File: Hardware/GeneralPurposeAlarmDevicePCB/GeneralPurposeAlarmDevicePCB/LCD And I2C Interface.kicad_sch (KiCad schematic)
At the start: 18 parts, among them Q301 BSS138, U301 PCF8574AT, U302 LCD_20x4_Character-GPAD_SCH_L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

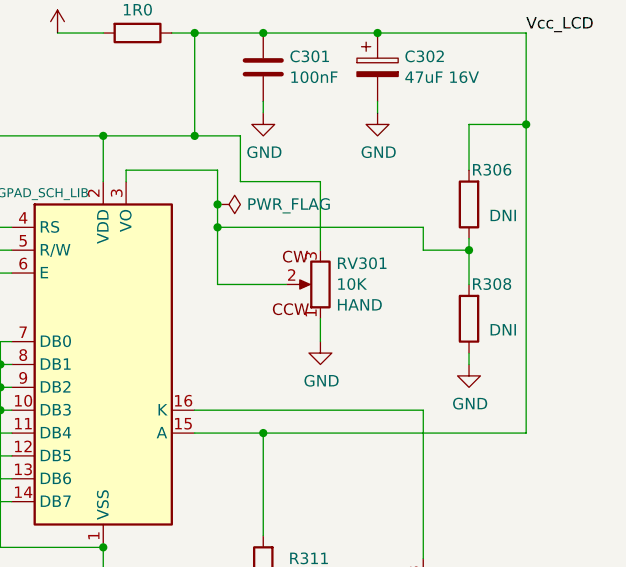
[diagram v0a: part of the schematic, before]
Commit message: Fix pot foot print, Add fifth mounting hole. Place all but UNO and test point.
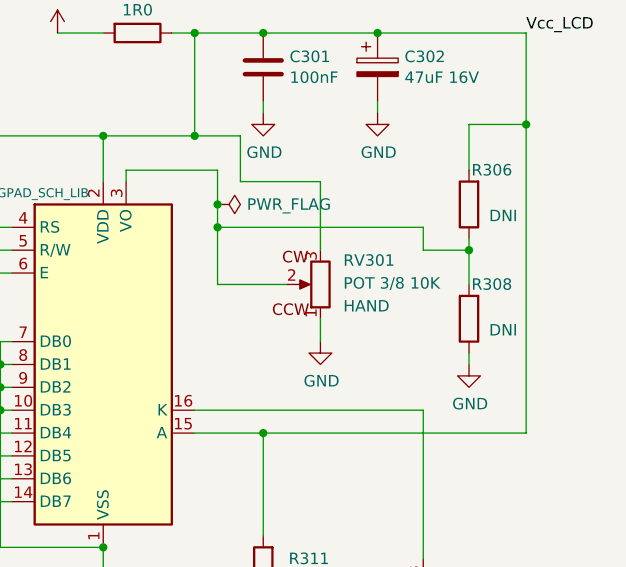
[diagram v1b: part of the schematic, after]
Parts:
- removed RV301: 10K, GeneralPurposeAlarmDevicePCB:Potentiometer_Bourns_3386P_Vertical, symbol GPAD_SCH_LIB:10K
- added RV301: POT 3/8 10K, GeneralPurposeAlarmDevicePCB:Potentiometer_Bourns_3386P_Vertical, symbol GPAD_SCH_LIB:POT 3/8 10K
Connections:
- net GND: now also RV301.1
- net Vcc_LCD: now also RV301.3
- net at R306.1, R308.2, U302.3 (VO): now also RV301.2
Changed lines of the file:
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@@
     (pin "1")
-  )
-  (symbol (lib_id "GPAD_SCH_LIB:10K") (at 209.55 68.58 180) (unit 1)
-    (in_bom yes) (on_board yes)
-    (property "Reference" "RV301" (id 0) (at 211.328 66.2686 0)
-      (effects (font (size 1.27 1.27)) (justify right))
-    )
-    (property "Value" "10K" (id 1) (at 211.328 68.58 0)
-      (effects (font (size 1.27 1.27)) (justify right))
-    )
-    (property "Footprint" "GeneralPurposeAlarmDevicePCB:Potentiometer_Bourns_3386P_Vertical" (id 2) (at 209.55 68.58 0)
-      (effects (font (size 1.27 1.27)) hide)
-    )
-    (property "Datasheet" "https://www.bourns.com/docs/Product-Datasheets/TC33.pdf" (id 3) (at 209.55 68.58 0)
-      (effects (font (size 1.27 1.27)) hide)
-    )
-    (property "Distributor 1" "JLCPCB" (id 4) (at 209.55 68.58 0)
-      (effects (font (size 1.27 1.27)) hide)
-    )
-    (property "Distributor 1 PN" "C58159" (id 5) (at 209.55 68.58 0)
-      (effects (font (size 1.27 1.27)) hide)
-    )
-    (property "Manufacturer" "BOURNS" (id 6) (at 209.55 68.58 0)
-      (effects (font (size 1.27 1.27)) hide)
-    )
-    (property "MPN" "3362P-1-103LF" (id 7) (at 209.55 68.58 0)
-      (effects (font (size 1.27 1.27)) hide)
-    )
-    (property "Assembly Type" "HAND" (id 8) (at 211.328 70.8914 0)
-      (effects (font (size 1.27 1.27)) (justify right))
-    )
-    (property "Manufacturier" "BOURNS" (id 9) (at 209.55 68.58 0)
-      (effects (font (size 1.27 1.27)) hide)
-    )
-    (pin "1")
-    (pin "2")
-    (pin "3")
   )
   (symbol (lib_id "power:PWR_FLAG") (at 167.64 49.53 0) (unit 1)
@@
     (pin "2")
   )
+  (symbol (lib_id "GPAD_SCH_LIB:POT 3/8 10K") (at 209.55 68.58 180) (unit 1)
+    (in_bom yes) (on_board yes) (fields_autoplaced)
+    (property "Reference" "RV301" (id 0) (at 212.09 65.9129 0)
+      (effects (font (size 1.27 1.27)) (justify right))
+    )
+    (property "Value" "POT 3/8 10K" (id 1) (at 212.09 68.4529 0)
+      (effects (font (size 1.27 1.27)) (justify right))
+    )
+    (property "Footprint" "GeneralPurposeAlarmDevicePCB:Potentiometer_Bourns_3386P_Vertical" (id 2) (at 209.55 68.58 0)
+      (effects (font (size 1.27 1.27)) hide)
+    )
+    (property "Datasheet" "https://www.bourns.com/docs/Product-Datasheets/3386.pdf" (id 3) (at 209.55 68.58 0)
+      (effects (font (size 1.27 1.27)) hide)
+    )
+    (property "Distributor 1" "JLCPCB" (id 4) (at 209.55 68.58 0)
+      (effects (font (size 1.27 1.27)) hide)
+    )
+    (property "Distributor 1 PN" "C116281" (id 5) (at 209.55 68.58 0)
+      (effects (font (size 1.27 1.27)) hide)
+    )
+    (property "Manufacturier" "BOURNS" (id 6) (at 209.55 68.58 0)
+      (effects (font (size 1.27 1.27)) hide)
+    )
+    (property "MPN" "3386P-1-103LF" (id 7) (at 209.55 68.58 0)
+      (effects (font (size 1.27 1.27)) hide)
+    )
+    (property "Assembly Type" "HAND" (id 8) (at 212.09 70.9929 0)
+      (effects (font (size 1.27 1.27)) (justify right))
+    )
+    (property "Distributor 2" "Digi-Key" (id 9) (at 209.55 68.58 0)
+      (effects (font (size 1.27 1.27)) hide)
+    )
+    (property "Distributor 2 PN" "3386P-103LF-ND" (id 10) (at 212.09 72.2629 0)
+      (effects (font (size 1.27 1.27)) (justify right) hide)
+    )
+    (property "Cost" "" (id 11) (at 209.55 68.58 0))
+    (pin "1")
+    (pin "2")
+    (pin "3")
+  )
   (symbol (lib_id "GPAD_SCH_LIB:LCD_20x4_Character-GPAD_SCH_LIB") (at 185.42 77.47 0) (unit 1)

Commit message: Delete lines related to the pot. The schematic now loads.
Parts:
- RV301: value POT 3/8 10K -> POT 0.375 10K; symbol GPAD_SCH_LIB:POT 3/8 10K -> GPAD_SCH_LIB:POT 0.375 10K
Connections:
- net GND: no longer RV301.1
- net Vcc_LCD: no longer RV301.3
- net at R306.1, R308.2, U302.3 (VO): no longer RV301.2
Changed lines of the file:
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@@
     (pin "2")
   )
-  (symbol (lib_id "GPAD_SCH_LIB:POT 3/8 10K") (at 209.55 68.58 180) (unit 1)
+  (symbol (lib_id "GPAD_SCH_LIB:POT 0.375 10K") (at 209.55 68.58 180) (unit 1)
     (in_bom yes) (on_board yes) (fields_autoplaced)
     (property "Reference" "RV301" (id 0) (at 212.09 65.9129 0)
       (effects (font (size 1.27 1.27)) (justify right))
     )
-    (property "Value" "POT 3/8 10K" (id 1) (at 212.09 68.4529 0)
+    (property "Value" "POT 0.375 10K" (id 1) (at 212.09 68.4529 0)
       (effects (font (size 1.27 1.27)) (justify right))
     )

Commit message: Re add the pot from the symbol library.
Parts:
- removed RV301: POT 0.375 10K, GeneralPurposeAlarmDevicePCB:Potentiometer_Bourns_3386P_Vertical, symbol GPAD_SCH_LIB:POT 0.375 10K
- added RV401: POT 0.375 10K, GeneralPurposeAlarmDevicePCB:Potentiometer_Bourns_3386P_Vertical, symbol GPAD_SCH_LIB:POT 0.375 10K
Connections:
- net GND: now also RV401.1
- net Vcc_LCD: now also RV401.3
- net at R306.1, R308.2, U302.3 (VO): now also RV401.2
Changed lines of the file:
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@@
     (pin "2")
-  )
-  (symbol (lib_id "GPAD_SCH_LIB:POT 0.375 10K") (at 209.55 68.58 180) (unit 1)
-    (in_bom yes) (on_board yes) (fields_autoplaced)
-    (property "Reference" "RV301" (id 0) (at 212.09 65.9129 0)
-      (effects (font (size 1.27 1.27)) (justify right))
-    )
-    (property "Value" "POT 0.375 10K" (id 1) (at 212.09 68.4529 0)
-      (effects (font (size 1.27 1.27)) (justify right))
-    )
-    (property "Footprint" "GeneralPurposeAlarmDevicePCB:Potentiometer_Bourns_3386P_Vertical" (id 2) (at 209.55 68.58 0)
-      (effects (font (size 1.27 1.27)) hide)
-    )
-    (property "Datasheet" "https://www.bourns.com/docs/Product-Datasheets/3386.pdf" (id 3) (at 209.55 68.58 0)
-      (effects (font (size 1.27 1.27)) hide)
-    )
-    (property "Distributor 1" "JLCPCB" (id 4) (at 209.55 68.58 0)
-      (effects (font (size 1.27 1.27)) hide)
-    )
-    (property "Distributor 1 PN" "C116281" (id 5) (at 209.55 68.58 0)
-      (effects (font (size 1.27 1.27)) hide)
-    )
-    (property "Manufacturier" "BOURNS" (id 6) (at 209.55 68.58 0)
-      (effects (font (size 1.27 1.27)) hide)
-    )
-    (property "MPN" "3386P-1-103LF" (id 7) (at 209.55 68.58 0)
-      (effects (font (size 1.27 1.27)) hide)
-    )
-    (property "Assembly Type" "HAND" (id 8) (at 212.09 70.9929 0)
-      (effects (font (size 1.27 1.27)) (justify right))
-    )
-    (property "Distributor 2" "Digi-Key" (id 9) (at 209.55 68.58 0)
-      (effects (font (size 1.27 1.27)) hide)
-    )
-    (property "Distributor 2 PN" "3386P-103LF-ND" (id 10) (at 212.09 72.2629 0)
-      (effects (font (size 1.27 1.27)) (justify right) hide)
-    )
-    (property "Cost" "" (id 11) (at 209.55 68.58 0))
-    (pin "1")
-    (pin "2")
-    (pin "3")
   )
   (symbol (lib_id "GPAD_SCH_LIB:LCD_20x4_Character-GPAD_SCH_LIB") (at 185.42 77.47 0) (unit 1)
@@
     (pin "9")
   )
+  (symbol (lib_id "GPAD_SCH_LIB:POT 0.375 10K") (at 209.55 68.58 180) (unit 1)
+    (in_bom yes) (on_board yes) (fields_autoplaced)
+    (property "Reference" "RV401" (id 0) (at 212.09 64.6429 0)
+      (effects (font (size 1.27 1.27)) (justify right))
+    )
+    (property "Value" "POT 0.375 10K" (id 1) (at 212.09 67.1829 0)
+      (effects (font (size 1.27 1.27)) (justify right))
+    )
+    (property "Footprint" "GeneralPurposeAlarmDevicePCB:Potentiometer_Bourns_3386P_Vertical" (id 2) (at 209.55 68.58 0)
+      (effects (font (size 1.27 1.27)) hide)
+    )
+    (property "Datasheet" "https://www.bourns.com/docs/Product-Datasheets/3386.pdf" (id 3) (at 209.55 68.58 0)
+      (effects (font (size 1.27 1.27)) hide)
+    )
+    (property "Distributor 1" "JLCPCB" (id 4) (at 209.55 68.58 0)
+      (effects (font (size 1.27 1.27)) hide)
+    )
+    (property "Distributor 1 PN" "C116281" (id 5) (at 209.55 68.58 0)
+      (effects (font (size 1.27 1.27)) hide)
+    )
+    (property "Manufacturier" "BOURNS" (id 6) (at 209.55 68.58 0)
+      (effects (font (size 1.27 1.27)) hide)
+    )
+    (property "MPN" "3386P-1-103LF" (id 7) (at 209.55 68.58 0)
+      (effects (font (size 1.27 1.27)) hide)
+    )
+    (property "Assembly Type" "HAND" (id 8) (at 212.09 69.7229 0)
+      (effects (font (size 1.27 1.27)) (justify right))
+    )
+    (property "Distributor 2" "Digi-Key" (id 9) (at 209.55 68.58 0)
+      (effects (font (size 1.27 1.27)) hide)
+    )
+    (property "Distributor 2 PN" "3386P-103LF-ND" (id 10) (at 212.09 72.2629 0)
+      (effects (font (size 1.27 1.27)) (justify right))
+    )
+    (property "Cost" "" (id 11) (at 209.55 68.58 0))
+    (pin "1")
+    (pin "2")
+    (pin "3")
+  )
 )

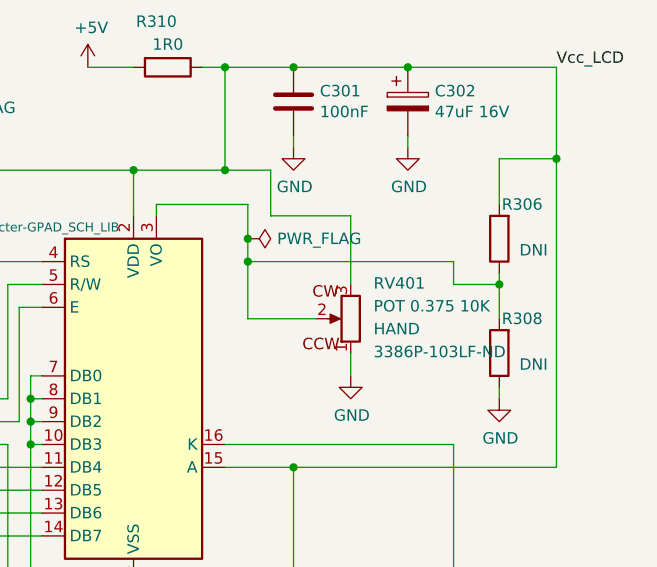
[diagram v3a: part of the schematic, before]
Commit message: Fixed library and schematic broken due to POT description including a "/" in symbol name.
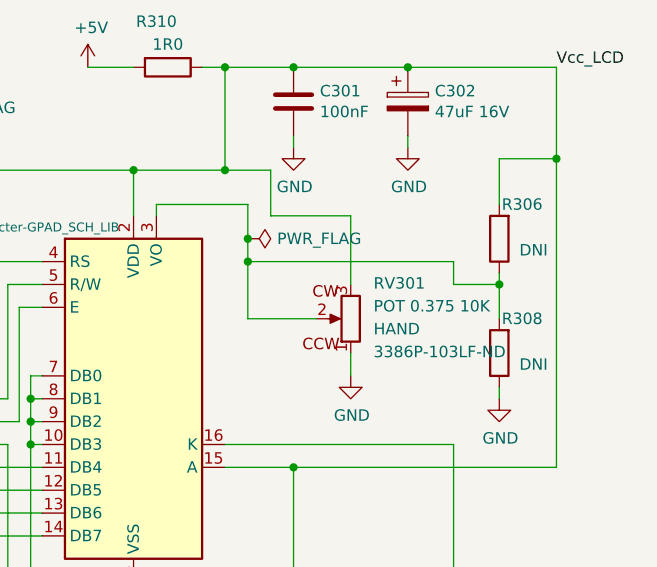
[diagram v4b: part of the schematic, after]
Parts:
- renumbered RV401 to RV301
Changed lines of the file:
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@@
   (symbol (lib_id "GPAD_SCH_LIB:POT 0.375 10K") (at 209.55 68.58 180) (unit 1)
     (in_bom yes) (on_board yes) (fields_autoplaced)
-    (property "Reference" "RV401" (id 0) (at 212.09 64.6429 0)
+    (property "Reference" "RV301" (id 0) (at 212.09 64.6429 0)
       (effects (font (size 1.27 1.27)) (justify right))
     )

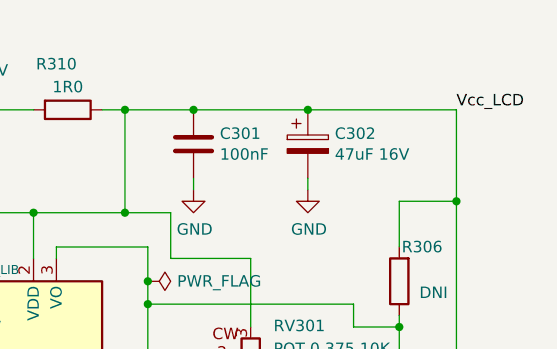
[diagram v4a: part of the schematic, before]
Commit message: Add 7805 alternative for linear regulator, Add test points on power supply nets, add MechanicalPartsPlacement.pdf.
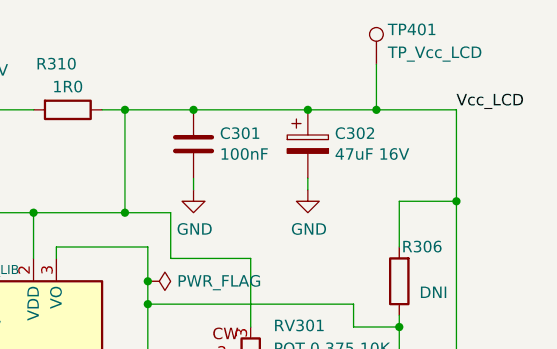
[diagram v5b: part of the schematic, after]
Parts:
- added TP401: TP_Vcc_LCD, TestPoint:TestPoint_Loop_D2.54mm_Drill1.5mm_Beaded, symbol Connector:TestPoint
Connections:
- net Vcc_LCD: now also TP401.1
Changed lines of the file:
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@@
   (junction (at 125.73 101.6) (diameter 0) (color 0 0 0 0)
   )
+  (junction (at 223.52 40.64) (diameter 0) (color 0 0 0 0)
+  )
   (junction (at 215.9 40.64) (diameter 0) (color 0 0 0 0)
   )
@@
     (stroke (width 0) (type default) (color 0 0 0 0))
   )
+  (wire (pts (xy 223.52 40.64) (xy 232.41 40.64))
+    (stroke (width 0) (type default) (color 0 0 0 0))
+  )
   (wire (pts (xy 185.42 52.07) (xy 185.42 57.15))
     (stroke (width 0) (type default) (color 0 0 0 0))
@@
     (stroke (width 0) (type default) (color 0 0 0 0))
   )
-  (wire (pts (xy 215.9 40.64) (xy 232.41 40.64))
+  (wire (pts (xy 215.9 40.64) (xy 223.52 40.64))
     (stroke (width 0) (type default) (color 0 0 0 0))
   )
@@
   )
   (wire (pts (xy 173.99 82.55) (xy 173.99 80.01))
+    (stroke (width 0) (type default) (color 0 0 0 0))
+  )
+  (wire (pts (xy 223.52 35.56) (xy 223.52 40.64))
     (stroke (width 0) (type default) (color 0 0 0 0))
   )
@@
     (pin "3")
   )
+  (symbol (lib_id "Connector:TestPoint") (at 223.52 35.56 0) (unit 1)
+    (in_bom yes) (on_board yes)
+    (property "Reference" "TP401" (id 0) (at 224.79 31.75 0)
+      (effects (font (size 1.27 1.27)) (justify left))
+    )
+    (property "Value" "TP_Vcc_LCD" (id 1) (at 224.79 34.29 0)
+      (effects (font (size 1.27 1.27)) (justify left))
+    )
+    (property "Footprint" "TestPoint:TestPoint_Loop_D2.54mm_Drill1.5mm_Beaded" (id 2) (at 228.6 35.56 0)
+      (effects (font (size 1.27 1.27)) hide)
+    )
+    (property "Datasheet" "~" (id 3) (at 228.6 35.56 0)
+      (effects (font (size 1.27 1.27)) hide)
+    )
+    (pin "1")
+  )
 )

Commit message: Change to LM7805 regulator. Delete the smaller more expensive SMT regulator.
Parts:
- RV301: Manufacturer (none) -> BOURNS; Manufacturer  (none) -> BOURNS; Manufacturier BOURNS -> (none)
- U302: Assembly Type (none) -> HAND; Distributor 1 Aliexpress -> (none); Distributor 1 PN https://www.aliexpress.com/item/3256803213374992.html -> (none); Distributor 2 Amazon -> (none); Distributor 2 PN https://www.amazon.com/GeeekPi-Interface-Adapter-Backlight-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 -> (none)
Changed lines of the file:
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@@
       (effects (font (size 1.27 1.27)) hide)
     )
-    (property "Distributor 1" "Aliexpress" (id 4) (at 157.988 94.996 0)
+    (property "Distributor 1" "" (id 4) (at 157.988 94.996 0)
       (effects (font (size 1.27 1.27)) hide)
     )
-    (property "Distributor 1 PN" "https://www.aliexpress.com/item/3256803213374992.html" (id 5) (at 182.88 97.536 0)
+    (property "Distributor 1 PN" "" (id 5) (at 182.88 97.536 0)
       (effects (font (size 1.27 1.27)) hide)
     )
-    (property "Distributor 2" "Amazon" (id 6) (at 156.972 100.584 0)
+    (property "Distributor 2" "" (id 6) (at 156.972 100.584 0)
       (effects (font (size 1.27 1.27)) hide)
     )
-    (property "Distributor 2 PN" "https://www.amazon.com/GeeekPi-Interface-Adapter-Backlight-Raspberry/dp/B07QLRD3TM/ref=sr_1_2" (id 7) (at 205.486 102.87 0)
+    (property "Distributor 2 PN" "" (id 7) (at 205.486 102.87 0)
+      (effects (font (size 1.27 1.27)) hide)
+    )
+    (property "Assembly Type" "HAND" (id 8) (at 185.42 77.47 0)
+      (effects (font (size 1.27 1.27)) hide)
+    )
+    (property "Cost" "" (id 9) (at 185.42 77.47 0)
+      (effects (font (size 1.27 1.27)) hide)
+    )
+    (property "Description" "" (id 10) (at 185.42 77.47 0)
+      (effects (font (size 1.27 1.27)) hide)
+    )
+    (property "MPN" "" (id 11) (at 185.42 77.47 0)
+      (effects (font (size 1.27 1.27)) hide)
+    )
+    (property "MPN " "" (id 12) (at 185.42 77.47 0)
+      (effects (font (size 1.27 1.27)) hide)
+    )
+    (property "Manufacturer" "" (id 13) (at 185.42 77.47 0)
+      (effects (font (size 1.27 1.27)) hide)
+    )
+    (property "Manufacturer " "" (id 14) (at 185.42 77.47 0)
       (effects (font (size 1.27 1.27)) hide)
     )
@@
       (effects (font (size 1.27 1.27)) hide)
     )
-    (property "Manufacturier" "BOURNS" (id 6) (at 209.55 68.58 0)
+    (property "Manufacturier" "" (id 6) (at 209.55 68.58 0)
       (effects (font (size 1.27 1.27)) hide)
     )
@@
     )
     (property "Cost" "" (id 11) (at 209.55 68.58 0))
+    (property "Manufacturer" "BOURNS" (id 12) (at 209.55 68.58 0)
+      (effects (font (size 1.27 1.27)) hide)
+    )
+    (property "Manufacturer " "BOURNS" (id 13) (at 209.55 68.58 0)
+      (effects (font (size 1.27 1.27)) hide)
+    )
     (pin "1")
     (pin "2")
